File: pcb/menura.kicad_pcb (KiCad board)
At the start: 2 copper layers, 123 x 97.2 mm, 56 parts, among them SW1 SW_Push, SW10 SW_Push, SW11 SW_Push, SW12 SW_Push, SW13 SW_Push, SW14 SW_Push, SW15 SW_Push, SW16 SW_Push, SW17 SW_Push, SW18 SW_Push, SW19 SW_Push, SW2 SW_Push, SW20 SW_Push, SW21 SW_Push, SW22 SW_Push, SW3 SW_Push, SW4 SW_Push, SW5 SW_Push, SW6 SW_Push, SW7 SW_Push, SW8 SW_Push, SW9 SW_Push

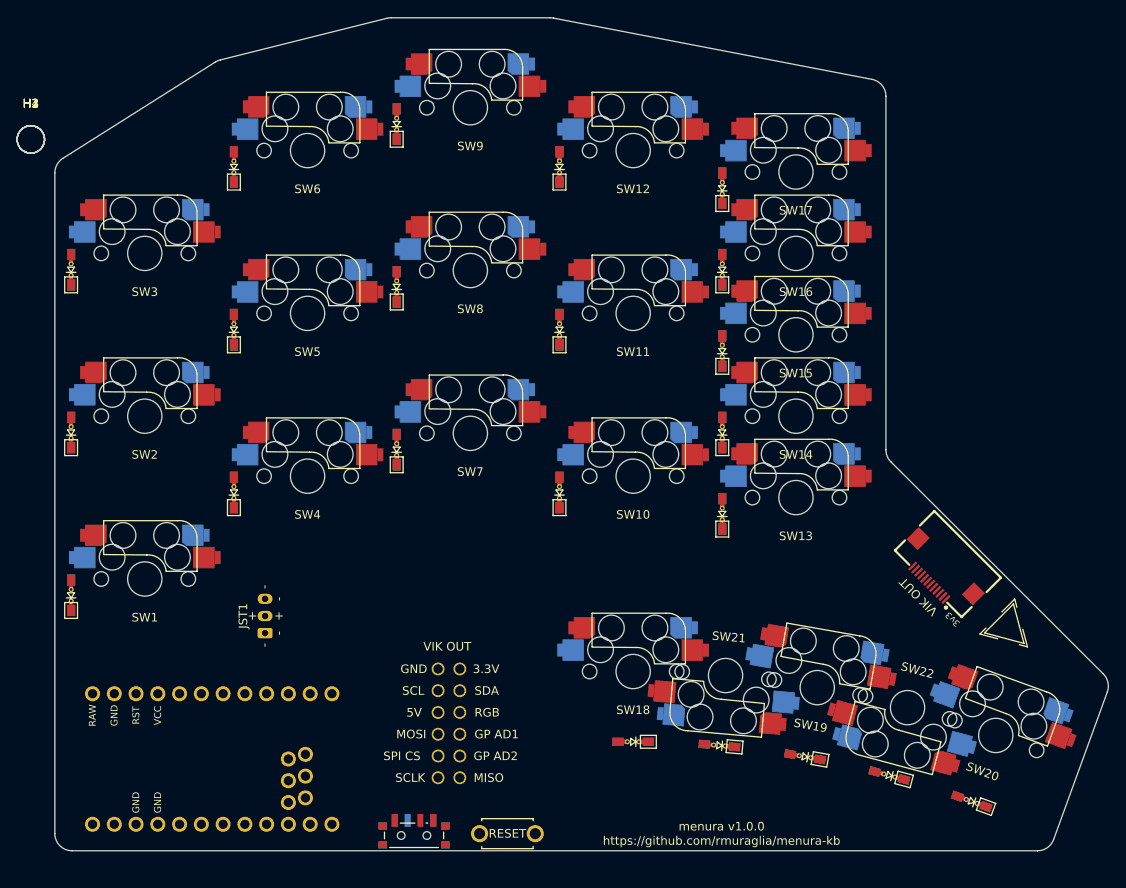
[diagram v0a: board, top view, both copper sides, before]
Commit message: holes
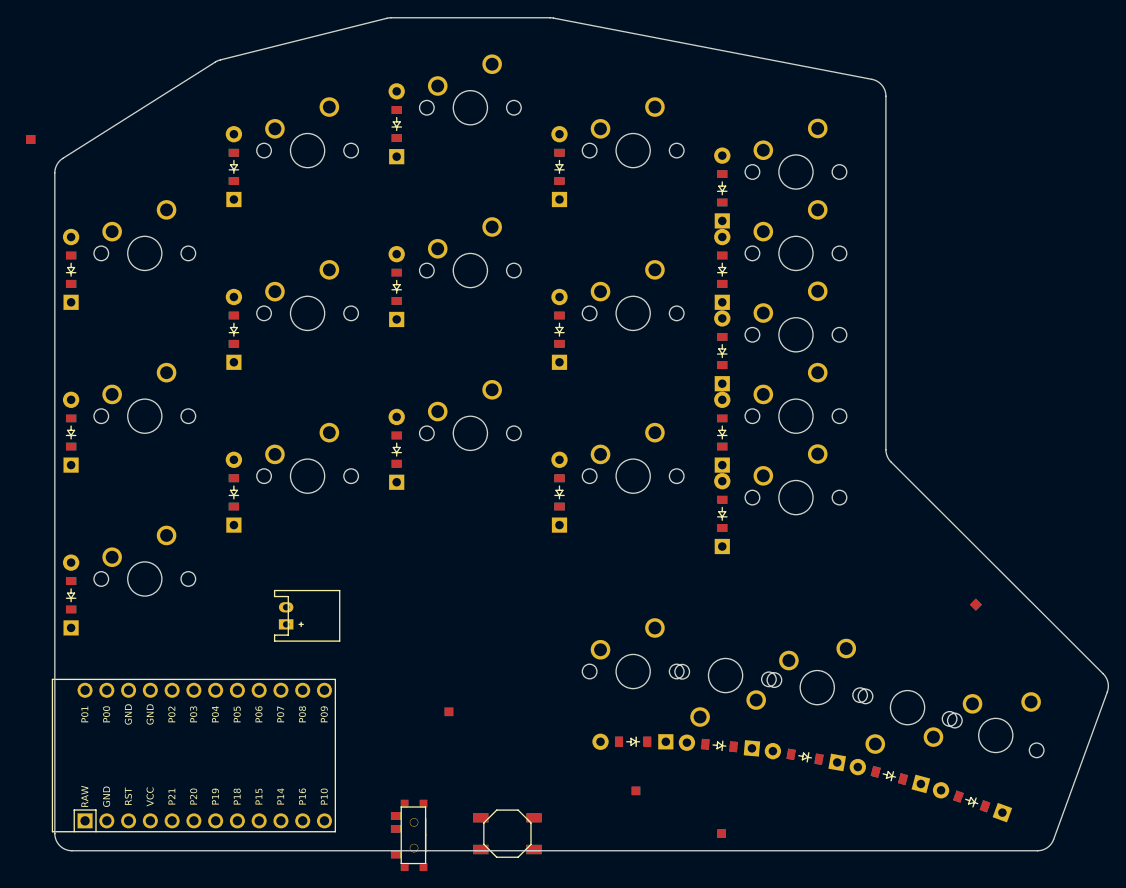
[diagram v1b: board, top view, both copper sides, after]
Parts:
- D1, D10, D11, D12, D13, D14, D15, D16, D17, D18, D19, D2, D20, D21, D22, D3, D4, D5, D6, D7, D8, D9: value 1N4148W -> (none); footprint quappo:Diode_SMD-reversible-urchin -> ComboDiode
- H1, H2, H3, H4: value MountingHole -> (none); footprint MountingHole:MountingHole_3.2mm_M3 -> SMDPad
- JST1: value Conn_01x03_Socket -> (none); footprint quappo:Connector_JST-PH-3prong -> JST_PH_S2B-PH-K_02x2.00mm_Angled
- LOGO1: value menura -> (none); footprint quappo:Logo_menura -> SMDPad
- LOGO2: value vik -> (none); footprint quappo:Logo_vik-small -> SMDPad
- MCU1: value N!N -> (none); footprint quappo:MCU_nice-nano -> ProMicro
- PWR1: value SW_SPDT -> (none); footprint quappo:Switch_power-reversible-kim -> E73:SPDT_C128955
- RSW1: value SW_Push -> (none); footprint quappo:Switch_reset-2pin -> E73:SW_TACT_ALPS_SKQGABE010
- SW1, SW10, SW11, SW12, SW13, SW14, SW15, SW16, SW17, SW18, SW19, SW2, SW20, SW21, SW22, SW3, SW4, SW5, SW6, SW7, SW8, SW9: value SW_Push -> (none); footprint quappo:Switch_MX-hotswap-reversible -> MX
- VIK1: value ~ -> (none); footprint quappo:Connector_vik-keyboard-horizontal -> SMDPad
- VIK2: value ~ -> (none); footprint quappo:Connector_vik-keyboard-throughhole -> SMDPad
- moved LOGO2 47.5 mm to (157.3, 124.7), turned to 360 degrees
- moved VIK1 5.66 mm to (197.0, 103.0)
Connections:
- D1 pad 1: row2 -> (no net)
- D1 pad 2: Net-(D1-A) -> (no net)
- D10 pad 1: row2 -> (no net)
- D10 pad 2: Net-(D10-A) -> (no net)
- D11 pad 1: row1 -> (no net)
- D11 pad 2: Net-(D11-A) -> (no net)
- D12 pad 1: row0 -> (no net)
- D12 pad 2: Net-(D12-A) -> (no net)
- D13 pad 1: row2 -> (no net)
- D13 pad 2: Net-(D13-A) -> (no net)
- D14 pad 1: row1 -> (no net)
- D14 pad 2: Net-(D14-A) -> (no net)
- D15 pad 1: row1 -> (no net)
- D15 pad 2: Net-(D15-A) -> (no net)
- D16 pad 1: row0 -> (no net)
- D16 pad 2: Net-(D16-A) -> (no net)
- D17 pad 1: row0 -> (no net)
- D17 pad 2: Net-(D17-A) -> (no net)
- D18 pad 1: row3 -> (no net)
- D18 pad 2: Net-(D18-A) -> (no net)
- D19 pad 1: row3 -> (no net)
- D19 pad 2: Net-(D19-A) -> (no net)
- D2 pad 1: row1 -> (no net)
- D2 pad 2: Net-(D2-A) -> (no net)
- D20 pad 1: row3 -> (no net)
- D20 pad 2: Net-(D20-A) -> (no net)
- D21 pad 1: row3 -> (no net)
- D21 pad 2: Net-(D21-A) -> (no net)
- D22 pad 1: row3 -> (no net)
- D22 pad 2: Net-(D22-A) -> (no net)
- D3 pad 1: row0 -> (no net)
- D3 pad 2: Net-(D3-A) -> (no net)
- D4 pad 1: row2 -> (no net)
- D4 pad 2: Net-(D4-A) -> (no net)
- D5 pad 1: row1 -> (no net)
- D5 pad 2: Net-(D5-A) -> (no net)
- D6 pad 1: row0 -> (no net)
- D6 pad 2: Net-(D6-A) -> (no net)
- D7 pad 1: row2 -> (no net)
- D7 pad 2: Net-(D7-A) -> (no net)
- D8 pad 1: row1 -> (no net)
- D8 pad 2: Net-(D8-A) -> (no net)
- D9 pad 1: row0 -> (no net)
- D9 pad 2: Net-(D9-A) -> (no net)
- JST1 pad 1: GND -> (no net)
- JST1 pad 2: Net-(JST1-Pin_2) -> (no net)
- MCU1 pad 1: unconnected-(MCU1-006-Pad1) -> RAW
- MCU1 pad 10: CS -> P14
- MCU1 pad 11: col4 -> P16
- MCU1 pad 12: row3 -> P10
- MCU1 pad 13: col3 -> P1
- MCU1 pad 14: col2 -> P0
- MCU1 pad 15: col1 -> GND
- MCU1 pad 16: col0 -> GND
- MCU1 pad 17: VIK_GPIO2 -> P2
- MCU1 pad 18: VIK_GPIO1 -> P3
- MCU1 pad 19: row2 -> P4
- MCU1 pad 2: row0 -> GND
- MCU1 pad 20: row1 -> P5
- MCU1 pad 21: +3.3V -> P6
- MCU1 pad 22: RST -> P7
- MCU1 pad 23: GND -> P8
- MCU1 pad 24: RAW -> P9
- MCU1 pad 3: GND -> RST
- MCU1 pad 4: GND -> VCC
- MCU1 pad 5: SDA -> P21
- MCU1 pad 6: SCL -> P20
- MCU1 pad 7: SCLK -> P19
- MCU1 pad 8: MISO -> P18
- MCU1 pad 9: MOSI -> P15
- PWR1 pad 1: RAW -> (no net)
- PWR1 pad 2: Net-(JST1-Pin_2) -> (no net)
- PWR1 pad 3: unconnected-(PWR1-C-Pad3)_0 -> (no net)
- RSW1 pad 1: GND -> (no net)
- RSW1 pad 2: RST -> (no net)
- SW1 pad 1: col0 -> (no net)
- SW1 pad 2: Net-(D1-A) -> (no net)
- SW10 pad 1: col3 -> (no net)
- SW10 pad 2: Net-(D10-A) -> (no net)
- SW11 pad 1: col3 -> (no net)
- SW11 pad 2: Net-(D11-A) -> (no net)
- SW12 pad 1: col3 -> (no net)
- SW12 pad 2: Net-(D12-A) -> (no net)
- SW13 pad 1: col4 -> (no net)
- SW13 pad 2: Net-(D13-A) -> (no net)
- SW14 pad 1: col4 -> (no net)
- SW14 pad 2: Net-(D14-A) -> (no net)
- SW15 pad 1: col4 -> (no net)
- SW15 pad 2: Net-(D15-A) -> (no net)
- SW16 pad 1: col4 -> (no net)
- SW16 pad 2: Net-(D16-A) -> (no net)
- SW17 pad 1: col4 -> (no net)
- SW17 pad 2: Net-(D17-A) -> (no net)
- SW18 pad 1: col2 -> (no net)
- SW18 pad 2: Net-(D18-A) -> (no net)
- SW19 pad 1: col3 -> (no net)
- SW19 pad 2: Net-(D19-A) -> (no net)
- SW2 pad 1: col0 -> (no net)
- SW2 pad 2: Net-(D2-A) -> (no net)
- SW20 pad 1: col4 -> (no net)
- SW20 pad 2: Net-(D20-A) -> (no net)
- SW21 pad 1: col2 -> (no net)
- SW21 pad 2: Net-(D21-A) -> (no net)
- SW22 pad 1: col3 -> (no net)
- SW22 pad 2: Net-(D22-A) -> (no net)
- SW3 pad 1: col0 -> (no net)
- SW3 pad 2: Net-(D3-A) -> (no net)
- SW4 pad 1: col1 -> (no net)
- SW4 pad 2: Net-(D4-A) -> (no net)
- SW5 pad 1: col1 -> (no net)
- SW5 pad 2: Net-(D5-A) -> (no net)
- SW6 pad 1: col1 -> (no net)
- SW6 pad 2: Net-(D6-A) -> (no net)
- SW7 pad 1: col2 -> (no net)
- SW7 pad 2: Net-(D7-A) -> (no net)
- SW8 pad 1: col2 -> (no net)
- SW8 pad 2: Net-(D8-A) -> (no net)
- SW9 pad 1: col2 -> (no net)
- SW9 pad 2: Net-(D9-A) -> (no net)
- VIK1 pad 1: +3.3V -> (no net)
- VIK2 pad 1: +3.3V -> (no net)
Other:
- net class Default added: clearance 0.2, trace_width 0.25, via_dia 0.8, via_drill 0.4
